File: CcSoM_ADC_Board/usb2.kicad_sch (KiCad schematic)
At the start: 12 parts, among them J18 USB_A, J19 USB_A, U10 USB3343

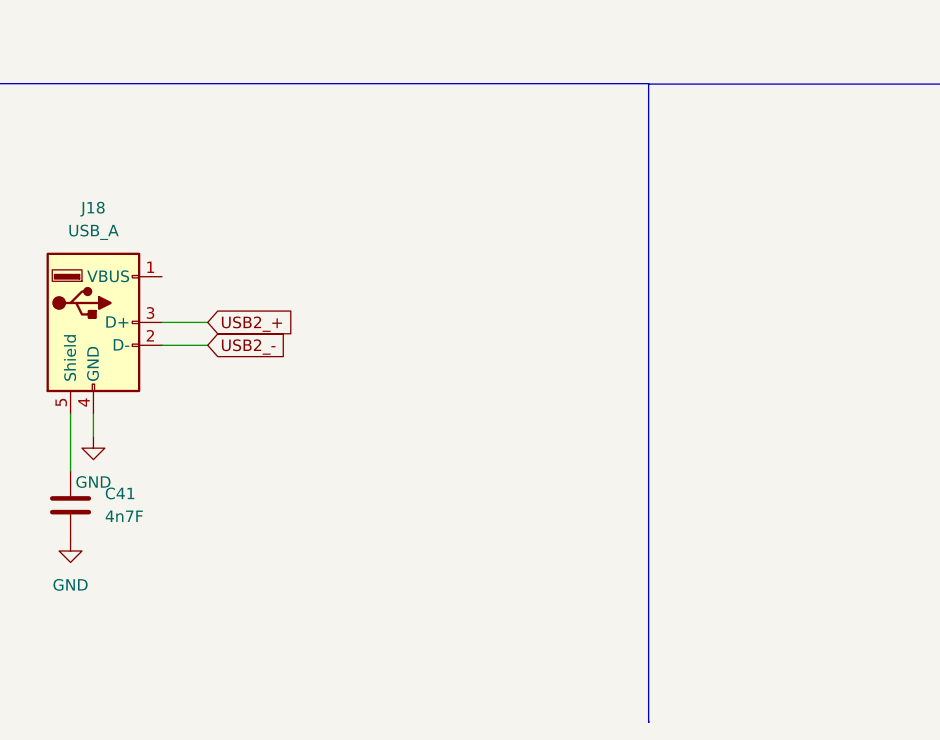
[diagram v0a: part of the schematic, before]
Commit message: last before rotating adc
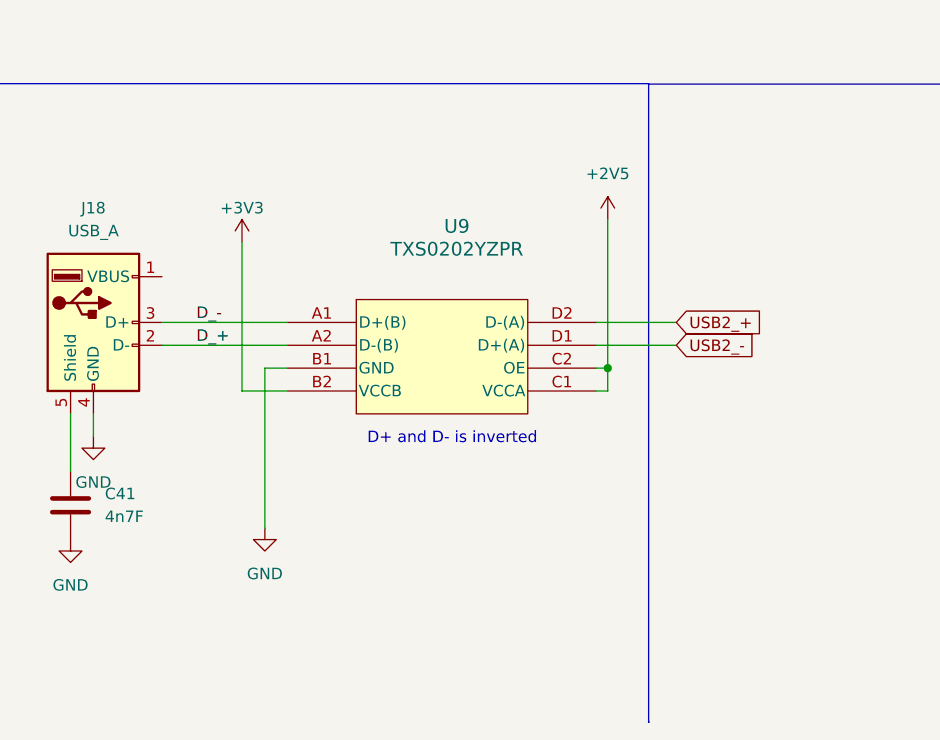
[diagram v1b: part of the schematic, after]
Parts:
- added U9: TXS0202YZPR, YZP8, symbol TXS0202YZPR:TXS0202YZPR
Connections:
- net +2V5: now also U9.C1 (VCCA), U9.C2 (OE)
- net GND: now also U9.B1 (GND)
- net USB2_+: now also U9.D2 (D-(A)); no longer J18.3 (D+)
- net USB2_-: now also U9.D1 (D+(A)); no longer J18.2 (D-)
- new net +3V3: U9.B2 (VCCB)
- new net D_+: J18.2 (D-), U9.A2 (D-(B))
- new net D_-: J18.3 (D+), U9.A1 (D+(B))
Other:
- note added: "D+ and D- is inverted"
